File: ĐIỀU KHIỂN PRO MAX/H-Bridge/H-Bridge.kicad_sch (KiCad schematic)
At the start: 11 parts, among them Q1 PMOS, Q2 PMOS, Q3 NMOS, Q4 NMOS

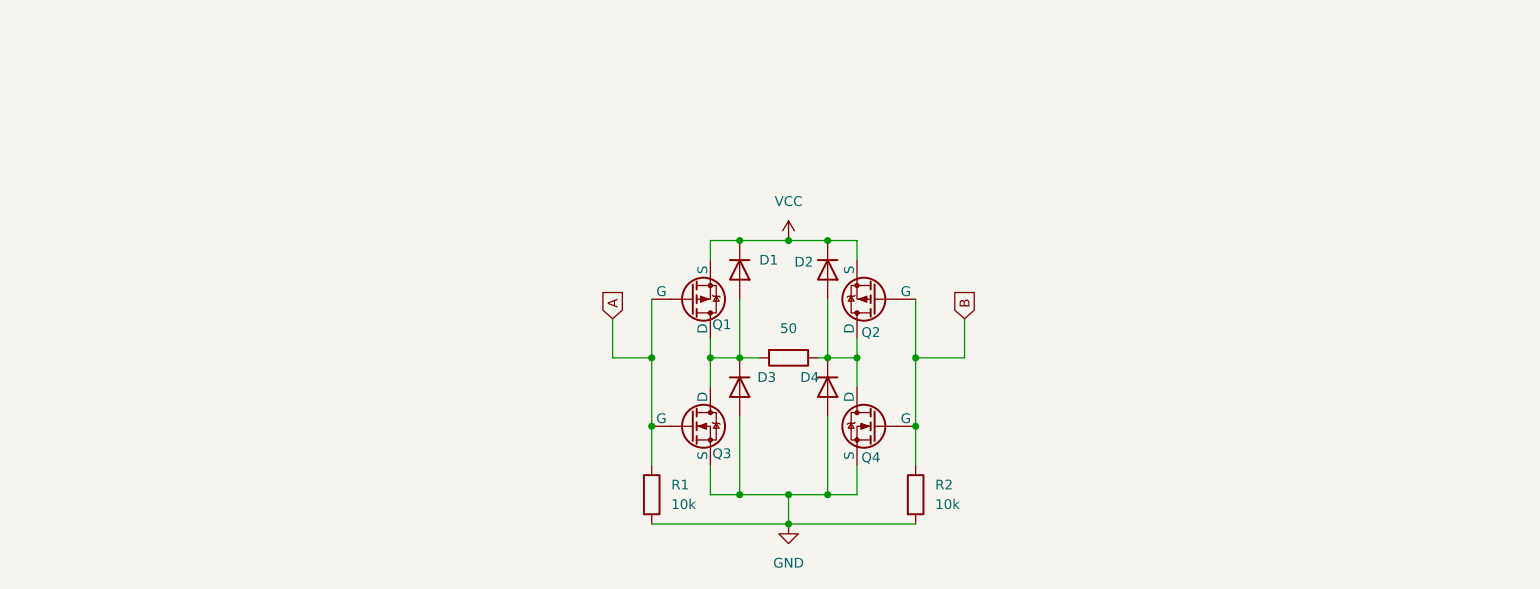
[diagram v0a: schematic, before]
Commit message: Push để pull về lại
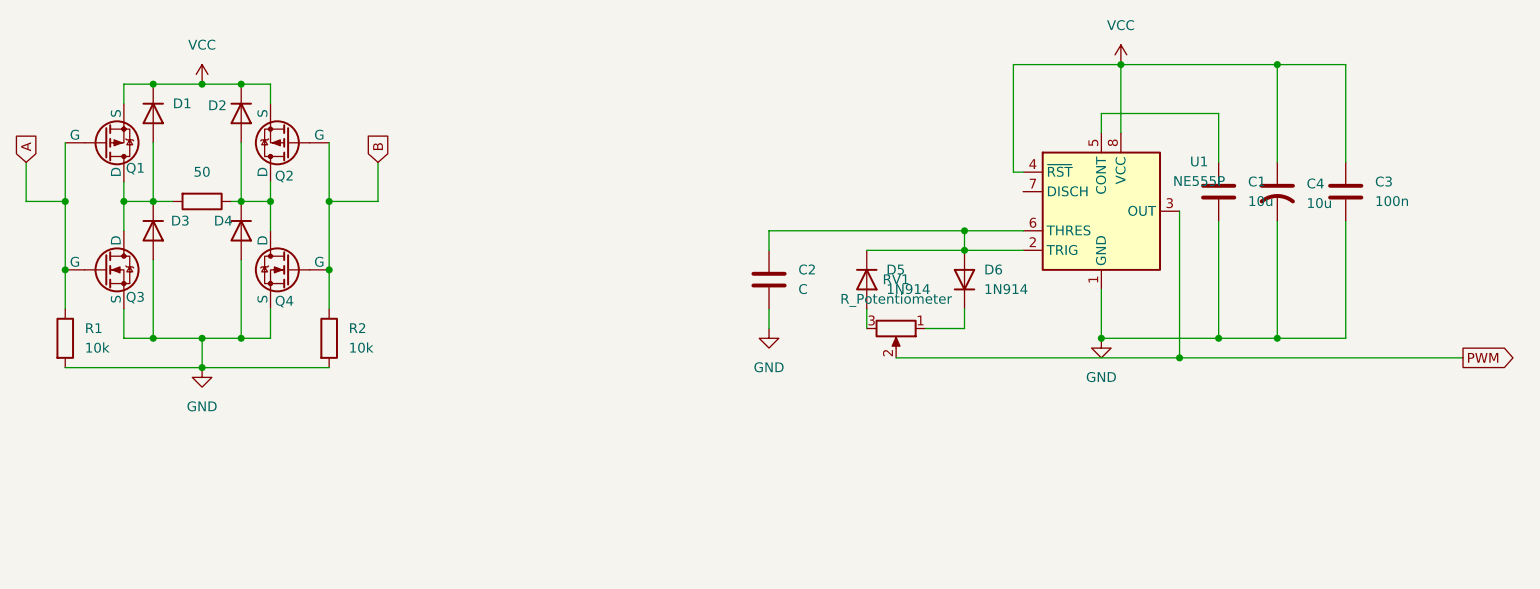
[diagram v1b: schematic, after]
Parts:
- added C1: 10u, symbol Device:C
- added C2: C, symbol Device:C
- added C3: 100n, symbol Device:C
- added C4: 10u, symbol Device:C_US
- added D5, D6: 1N914, Diode_THT:D_DO-35_SOD27_P7.62mm_Horizontal, symbol Diode:1N914
- added RV1: R_Potentiometer, symbol Device:R_Potentiometer
- added U1: NE555P, Package_DIP:DIP-8_W7.62mm, symbol Timer:NE555P
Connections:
- net GND: now also C1.2, C2.2, C3.2, C4.2, U1.1 (GND)
- net VCC: now also C3.1, C4.1, U1.4 (~{RST}), U1.8 (VCC)
- new net: D6.1 (K), RV1.1
- new net: C2.1, D5.1 (K), D6.2 (A), U1.2 (TRIG), U1.6 (THRES)
- new net: D5.2 (A), RV1.3
- new net: C1.1, U1.5 (CONT)
- new net PWM: RV1.2, U1.3 (OUT)
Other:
- moved on the sheet: D1, D2, D3, D4, Q1, Q2, Q3, Q4, R1, R2
